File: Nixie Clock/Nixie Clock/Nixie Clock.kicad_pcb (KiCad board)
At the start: 2 copper layers, 150 x 104 mm, 67 parts, among them J1 PJ-202A, J2 Conn_01x05_Male, Q1 MPSA55, SW1 1825910-2, U1 LM1086IT-5.0, U10 PIC16F15325-I/P, U2 MC34063AP, U3 IRF630, U4 TPIC6595N, U5 TPIC6595N, U6 TPIC6595N, U7 TPIC6595N, U8 TPIC6595N, U9 TPIC6595N, Y1 12.288MHz

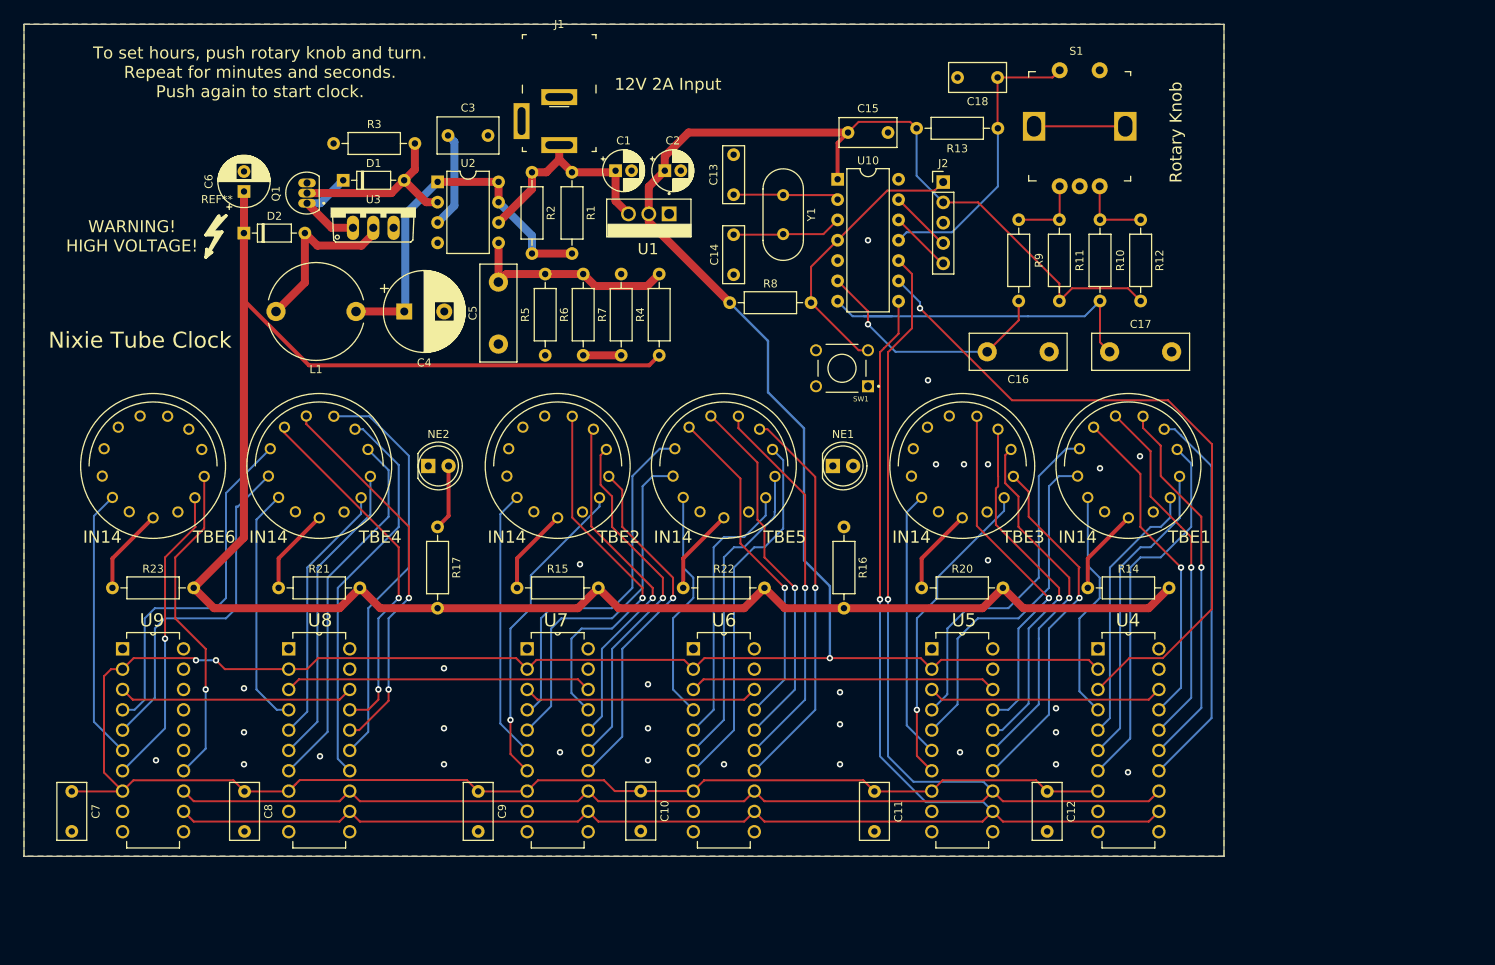
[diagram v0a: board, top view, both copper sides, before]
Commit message: Nixie
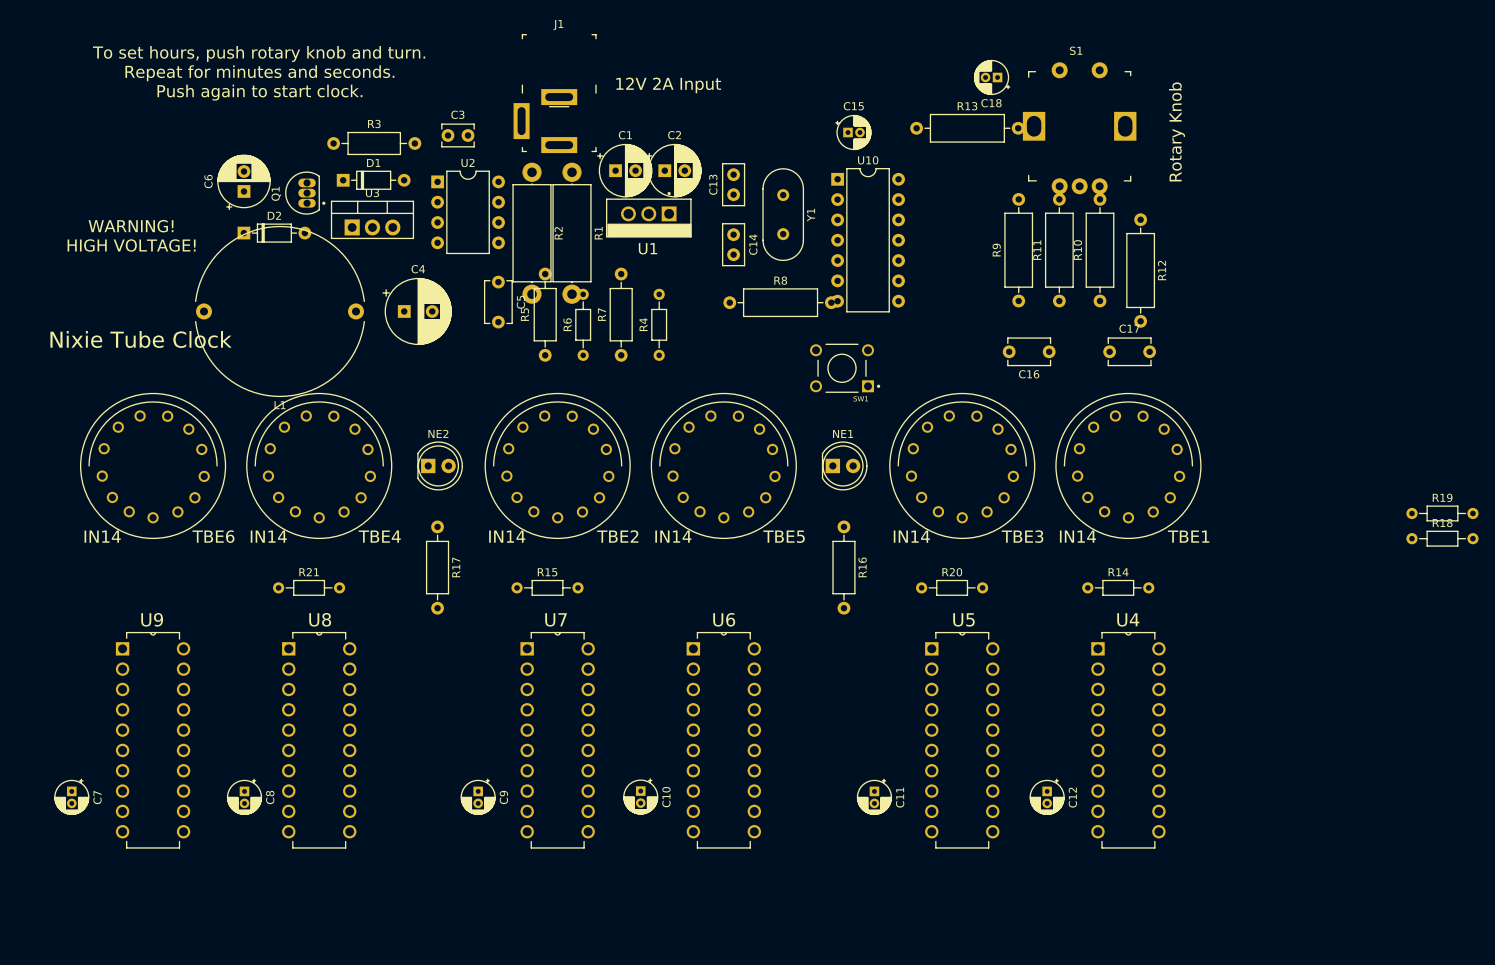
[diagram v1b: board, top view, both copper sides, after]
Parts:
- removed J2: Conn_01x05_Male, Connector_PinHeader_2.54mm:PinHeader_1x05_P2.54mm_Vertical
- removed R22, R23: 14k, Resistor_THT:R_Axial_DIN0207_L6.3mm_D2.5mm_P10.16mm_Horizontal
- removed REF**: Symbol_Highvoltage_Type1_CopperTop_Small, Symbol:Symbol_Highvoltage_Type1_CopperTop_Small
- added R18: 14k, Resistor_THT:R_Axial_DIN0204_L3.6mm_D1.6mm_P7.62mm_Horizontal, F.Cu at (243.5, 101.8)
- added R19: 14k, Resistor_THT:R_Axial_DIN0204_L3.6mm_D1.6mm_P7.62mm_Horizontal, F.Cu at (243.5, 98.7)
- C1, C2: footprint Capacitor_THT:CP_Radial_D5.0mm_P2.00mm -> Capacitor_THT:CP_Radial_D6.3mm_P2.50mm
- C10, C11, C12, C15, C18, C7, C8, C9: footprint Capacitor_THT:C_Rect_L7.0mm_W3.5mm_P5.00mm -> Capacitor_THT:CP_Radial_D4.0mm_P1.50mm
- C13, C14: footprint Capacitor_THT:C_Rect_L7.0mm_W2.5mm_P5.00mm -> Capacitor_THT:C_Disc_D5.0mm_W2.5mm_P2.50mm
- C16, C17, C5: footprint Capacitor_THT:C_Disc_D12.0mm_W4.4mm_P7.75mm -> Capacitor_THT:C_Disc_D5.1mm_W3.2mm_P5.00mm
- C3: footprint Capacitor_THT:C_Disc_D7.5mm_W4.4mm_P5.00mm -> Capacitor_THT:C_Disc_D3.8mm_W2.6mm_P2.50mm
- C4: footprint Capacitor_THT:CP_Radial_D10.0mm_P5.00mm -> Capacitor_THT:CP_Radial_D8.0mm_P3.50mm
- L1: footprint Inductor_THT:L_Radial_D12.0mm_P10.00mm_Neosid_SD12_style1 -> Inductor_THT:L_Radial_D21.0mm_P19.00mm
- R1, R2: footprint Resistor_THT:R_Axial_DIN0207_L6.3mm_D2.5mm_P10.16mm_Horizontal -> Resistor_THT:R_Axial_DIN0414_L11.9mm_D4.5mm_P15.24mm_Horizontal
- R10, R11, R12, R13, R8, R9: footprint Resistor_THT:R_Axial_DIN0207_L6.3mm_D2.5mm_P10.16mm_Horizontal -> Resistor_THT:R_Axial_DIN0309_L9.0mm_D3.2mm_P12.70mm_Horizontal
- R14, R15, R20, R21, R4, R6: footprint Resistor_THT:R_Axial_DIN0207_L6.3mm_D2.5mm_P10.16mm_Horizontal -> Resistor_THT:R_Axial_DIN0204_L3.6mm_D1.6mm_P7.62mm_Horizontal
- U3: footprint IRF630:TO220V -> Package_TO_SOT_THT:TO-220-3_Vertical
- moved U3 3.64 mm to (111.0, 62.9)
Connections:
- R11 pad 1: +5V -> Net-(R11-Pad1)
- R11 pad 2: Net-(R11-Pad2) -> +5V
- R12 pad 1: Net-(R10-Pad2) -> +5V
- R12 pad 2: +5V -> Net-(R10-Pad2)
- R13 pad 1: +5V -> /Microcontroller/Rotary Button
- R13 pad 2: /Microcontroller/Rotary Button -> +5V
- R9 pad 2: Net-(R11-Pad2) -> Net-(R11-Pad1)
- S1 pad A: Net-(R11-Pad2) -> Net-(R11-Pad1)
- TBE3 pad 1: Net-(R20-Pad1) -> Net-(R18-Pad1)
- TBE4 pad 1: Net-(R21-Pad1) -> Net-(R19-Pad1)
- TBE5 pad 1: Net-(R22-Pad1) -> Net-(R20-Pad1)
- TBE6 pad 1: Net-(R23-Pad1) -> Net-(R21-Pad1)
- U10 pad 12: /Microcontroller/Program Clock -> unconnected-(U10-Pad12)
- U10 pad 13: /Microcontroller/Program Data -> unconnected-(U10-Pad13)
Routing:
- net +5V: track 436.4 -> 0.00 mm, vias 3 -> 0
- net VDC: track 248.8 -> 0.00 mm
- net /Shift Clock: track 206.0 -> 0.00 mm, vias 1 -> 0
- net /Data Latch: track 202.0 -> 0.00 mm, vias 1 -> 0
- net /Data Output: track 87.1 -> 0.00 mm, vias 1 -> 0
- net /Tube_5_Digit_5: track 51.3 -> 0.00 mm
- net /Tube_5_Digit_4: track 49.3 -> 0.00 mm
- net /Tube_3_Digit_4: track 49.3 -> 0.00 mm, vias 1 -> 0
- net /Tube_1_Digit_4: track 48.6 -> 0.00 mm
- net /Tube_5_Digit_6: track 48.3 -> 0.00 mm, vias 2 -> 0
- net /Tube_3_Digit_5: track 47.9 -> 0.00 mm, vias 1 -> 0
- net Net-(C4-Pad1): track 47.3 -> 0.00 mm
- net /Tube_1_Digit_3: track 47.2 -> 0.00 mm
- net /Tube_4_Digit_5: track 47.1 -> 0.00 mm, vias 1 -> 0
- net /Tube_1_Digit_5: track 47.0 -> 0.00 mm, vias 1 -> 0
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- removed copper zone on B.Cu, net GND
- removed copper zone on F.Cu, net GND
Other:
- board outline removed

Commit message: Added additional parts
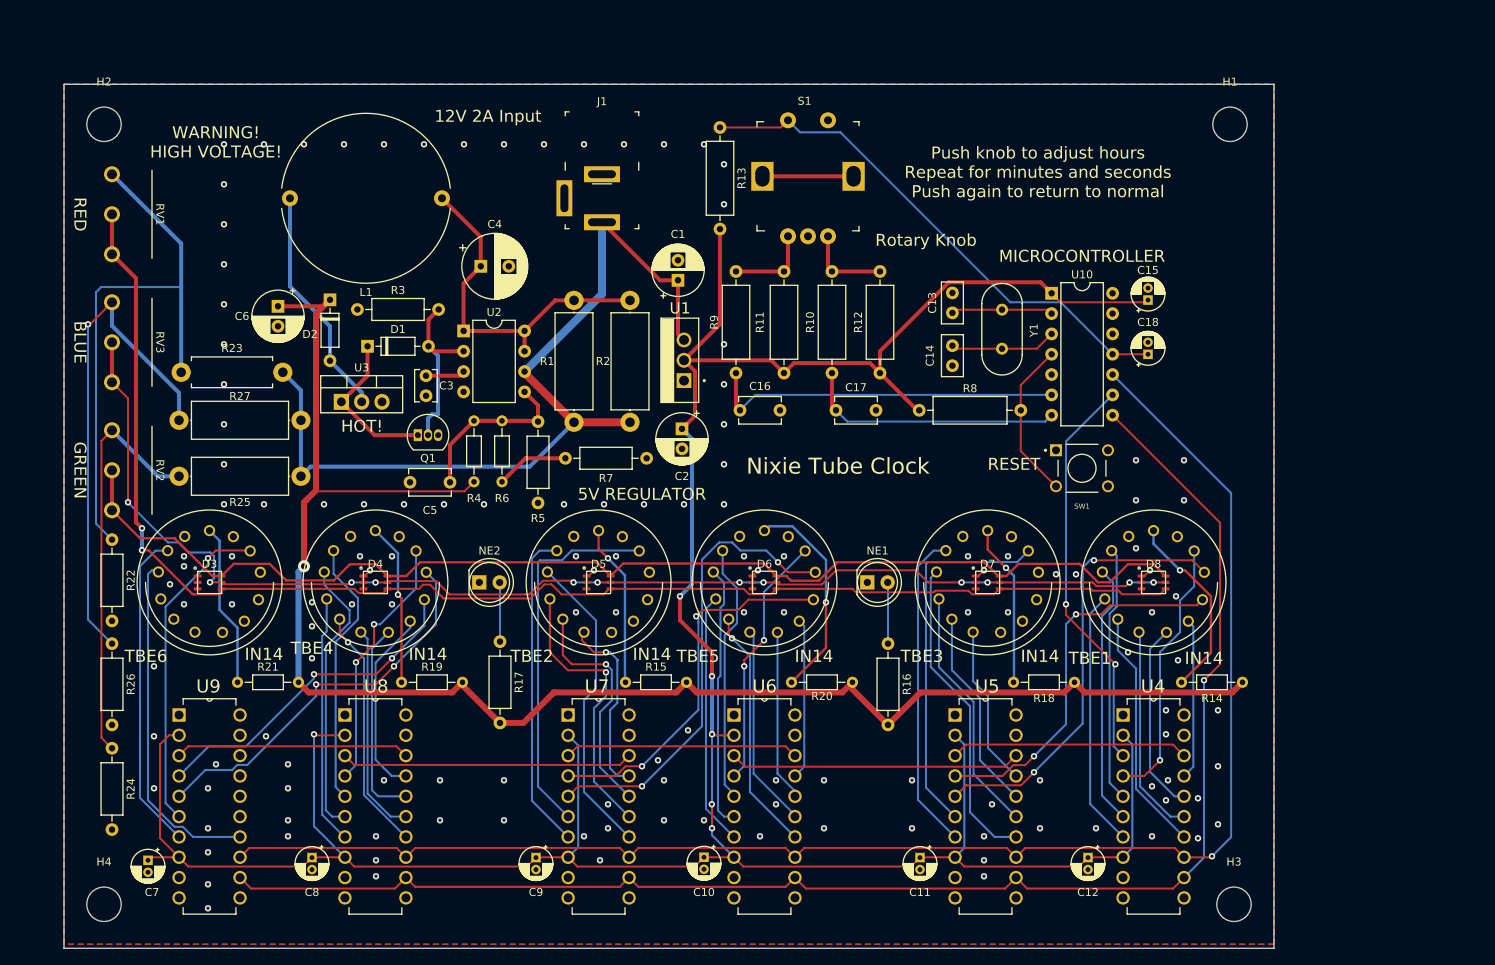
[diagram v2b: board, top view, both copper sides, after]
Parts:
- added D3: LED_RGB, CLY6D-FKC-CK1N1D1BB7D3D3:CLY6D-FKC-CK1N1D1BB7D3D3, F.Cu at (93.2, 107.3)
- added D4: LED_RGB, CLY6D-FKC-CK1N1D1BB7D3D3:CLY6D-FKC-CK1N1D1BB7D3D3, F.Cu at (113.9, 107.3)
- added D5: LED_RGB, CLY6D-FKC-CK1N1D1BB7D3D3:CLY6D-FKC-CK1N1D1BB7D3D3, F.Cu at (141.8, 107.3)
- added D6: LED_RGB, CLY6D-FKC-CK1N1D1BB7D3D3:CLY6D-FKC-CK1N1D1BB7D3D3, F.Cu at (162.6, 107.3)
- added D7: LED_RGB, CLY6D-FKC-CK1N1D1BB7D3D3:CLY6D-FKC-CK1N1D1BB7D3D3, F.Cu at (190.5, 107.3)
- added D8: LED_RGB, CLY6D-FKC-CK1N1D1BB7D3D3:CLY6D-FKC-CK1N1D1BB7D3D3, F.Cu at (211.2, 107.3)
- added H1: MountingHole, MountingHole:MountingHole_4.3mm_M4, F.Cu at (220.8, 50.0)
- added H2: MountingHole, MountingHole:MountingHole_4.3mm_M4, F.Cu at (80.0, 50.0)
- added H3: MountingHole, MountingHole:MountingHole_4.3mm_M4, F.Cu at (221.2, 147.5)
- added H4: MountingHole, MountingHole:MountingHole_4.3mm_M4, F.Cu at (80.0, 147.5)
- added R22: Resistor_THT:R_Axial_DIN0207_L6.3mm_D2.5mm_P10.16mm_Horizon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, Resistor_THT:R_Axial_DIN0207_L6.3mm_D2.5mm_P10.16mm_Horizontal, F.Cu at (81.0, 101.9)
- added R23: 110, Resistor_THT:R_Axial_DIN0411_L9.9mm_D3.6mm_P12.70mm_Horizontal, F.Cu at (102.3, 81.0)
- added R24: Resistor_THT:R_Axial_DIN0207_L6.3mm_D2.5mm_P10.16mm_Horizon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, Resistor_THT:R_Axial_DIN0207_L6.3mm_D2.5mm_P10.16mm_Horizontal, F.Cu at (81.0, 128.0)
- added R25: 150, Resistor_THT:R_Axial_DIN0414_L11.9mm_D4.5mm_P15.24mm_Horizontal, F.Cu at (104.6, 94.0)
- added R26: Resistor_THT:R_Axial_DIN0207_L6.3mm_D2.5mm_P10.16mm_Horizon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, Resistor_THT:R_Axial_DIN0207_L6.3mm_D2.5mm_P10.16mm_Horizontal, F.Cu at (81.0, 114.9)
- added R27: 150, Resistor_THT:R_Axial_DIN0414_L11.9mm_D4.5mm_P15.24mm_Horizontal, F.Cu at (104.6, 87.0)
- added RV1: 10K, WH148:WH148, F.Cu at (81.0, 61.2)
- added RV2: 10K, WH148:WH148, F.Cu at (81.0, 93.2)
- added RV3: 10K, WH148:WH148, F.Cu at (81.0, 77.2)
- Q1: footprint MPSA55:TO92127P520H787-3 -> Package_TO_SOT_THT:TO-92_Inline
- moved R19 128.1 mm to (117.2, 119.8)
- moved R18 52.9 mm to (193.7, 119.8)
- moved C15 43.0 mm to (210.5, 72.0), turned to 90 degrees
- moved C18 39.4 mm to (210.5, 78.8), turned to 90 degrees
- moved R12 37.8 mm to (177.0, 81.1), turned to 90 degrees
- moved R9 36.5 mm to (159.0, 81.1)
- moved C17 35.0 mm to (171.5, 85.8)
- moved R10 34.7 mm to (171.0, 81.1)
- moved R11 34.6 mm to (165.0, 68.4), turned to -90 degrees
- moved S1 34.5 mm to (162.3, 56.5)
- moved C16 34.4 mm to (164.5, 85.8)
- moved R2 33.6 mm to (145.8, 87.2), turned to 90 degrees
- moved Q1 33.3 mm to (119.2, 88.9), turned to 0 degrees
- moved C2 32.3 mm to (152.2, 88.1), turned to -90 degrees
- moved R1 31.3 mm to (138.8, 87.2), turned to 90 degrees
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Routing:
- net +5V: track 0.00 -> 376.8 mm, vias 0 -> 6
- net VDC: track 0.00 -> 207.1 mm, vias 0 -> 1
- net /Shift Clock: track 0.00 -> 193.7 mm, vias 0 -> 1
- net /Data Latch: track 0.00 -> 188.6 mm, vias 0 -> 1
- net /LEDS/RED: track 0.00 -> 178.8 mm, vias 0 -> 2
- net /LEDS/GRN: track 0.00 -> 160.9 mm, vias 0 -> 12
- net /LEDS/BLU: track 0.00 -> 150.9 mm
- net +12V: track 0.00 -> 109.7 mm
- net Net-(R22-Pad1): track 0.00 -> 71.0 mm
- net /Microcontroller/Rotary Button: track 0.00 -> 66.0 mm
- net Net-(R26-Pad1): track 0.00 -> 63.5 mm, vias 0 -> 1
- net /Tube_3_Digit_9: track 0.00 -> 57.8 mm, vias 0 -> 2
- net /Tube_1_Digit_9: track 0.00 -> 55.4 mm, vias 0 -> 2
- net Net-(R24-Pad1): track 0.00 -> 51.6 mm
- net /Data Output: track 0.00 -> 50.6 mm, vias 0 -> 2
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- added copper zone on B.Cu, net GND
- added copper zone on F.Cu, net GND
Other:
- board outline added: 151.2 x 108 mm
- board text added: "5V REGULATOR"
- board text added: "BLUE"
- board text added: "GREEN"
- board text added: "HOT!"
- board text added: "MICROCONTROLLER"
- board text added: "Push knob to adjust hours Repeat for minutes and seconds Push again to return to normal"
- board text added: "RED"
- board text added: "RESET"
- board text removed: "To set hours, push rotary knob and turn. Repeat for minutes and seconds. Push again to start clock."
